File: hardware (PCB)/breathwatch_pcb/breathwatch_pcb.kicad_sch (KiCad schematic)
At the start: 7 parts, among them J1 Conn_01x08_Socket, J2 Conn_01x08_Socket, J3 Conn_01x04_Socket, J4 USB_A, Q1 AO3401A

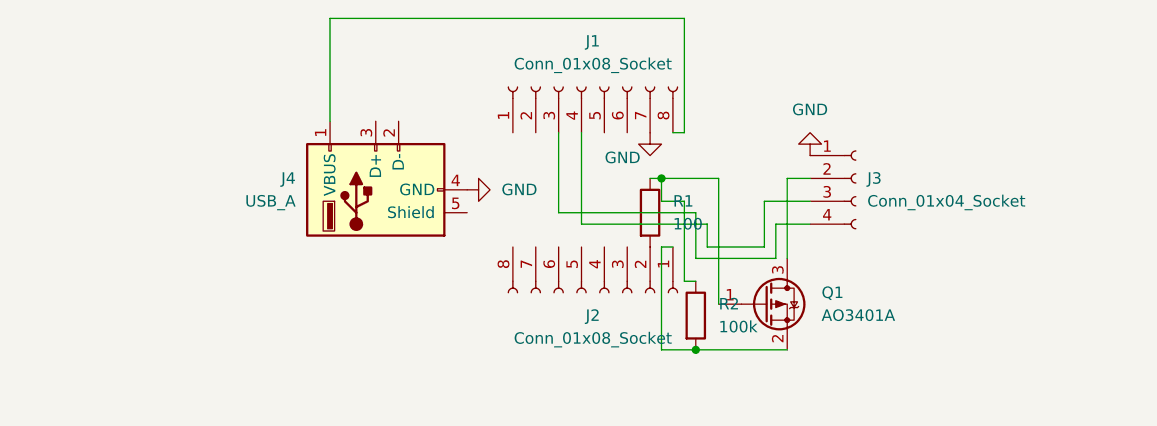
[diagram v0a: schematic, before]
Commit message: fixed a few things (PCB, Schematic)
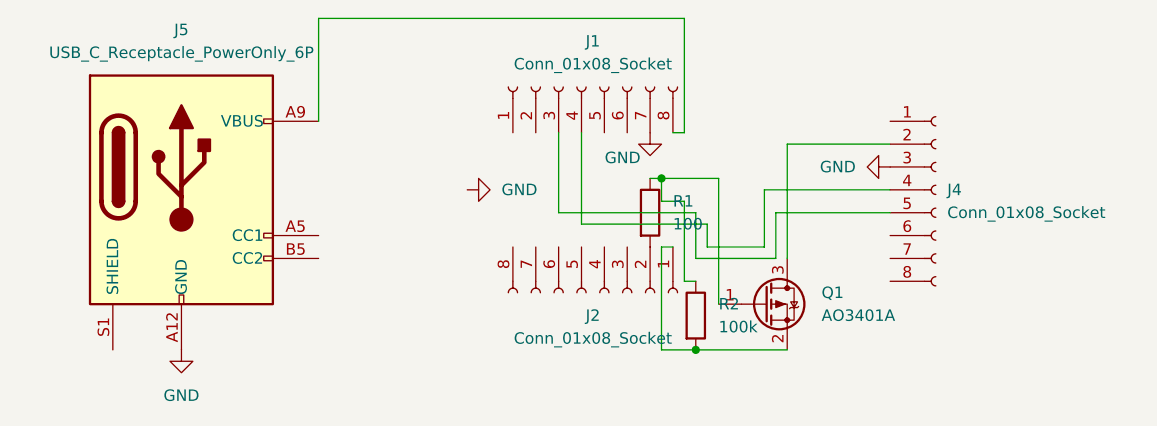
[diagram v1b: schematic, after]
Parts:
- removed J3: Conn_01x04_Socket, Connector_PinHeader_2.54mm:PinHeader_1x04_P2.54mm_Vertical, symbol Connector:Conn_01x04_Socket
- removed J4: USB_A, Connector_USB:USB_A_CNCTech_1001-011-01101_Horizontal, symbol Connector:USB_A
- added J4: Conn_01x08_Socket, Connector_PinSocket_2.54mm:PinSocket_1x08_P2.54mm_Vertical_SMD_Pin1Right, symbol Connector:Conn_01x08_Socket
- added J5: USB_C_Receptacle_PowerOnly_6P, Connector_USB:USB_C_Receptacle_GCT_USB4125-xx-x_6P_TopMnt_Horizontal, symbol Connector:USB_C_Receptacle_PowerOnly_6P
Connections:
- net GND: now also J4.3 (Pin_3), J5.A12 (GND), J5.B12 (GND)
- net at J1.3 (Pin_3): now also J4.5 (Pin_5)
- net at J1.4 (Pin_4): now also J4.4 (Pin_4)
- net at J1.8 (Pin_8): now also J5.A9 (VBUS), J5.B9 (VBUS)
- net at Q1.3 (D): now also J4.2 (Pin_2)
